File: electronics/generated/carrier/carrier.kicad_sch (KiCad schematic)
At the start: 11 parts, among them J1 EXTERNAL_3V3_CURRENT_LIMITED, J2 SPI_BANK_0, J3 SPI_BANK_1, J4 SPI_BANK_2, J5 SPI_BANK_3, J6 ADXL355_3V3_MODULE, J7 ODOMETER_3V3_ONLY, U1 Raspberry_Pi_Pico_USB_powered

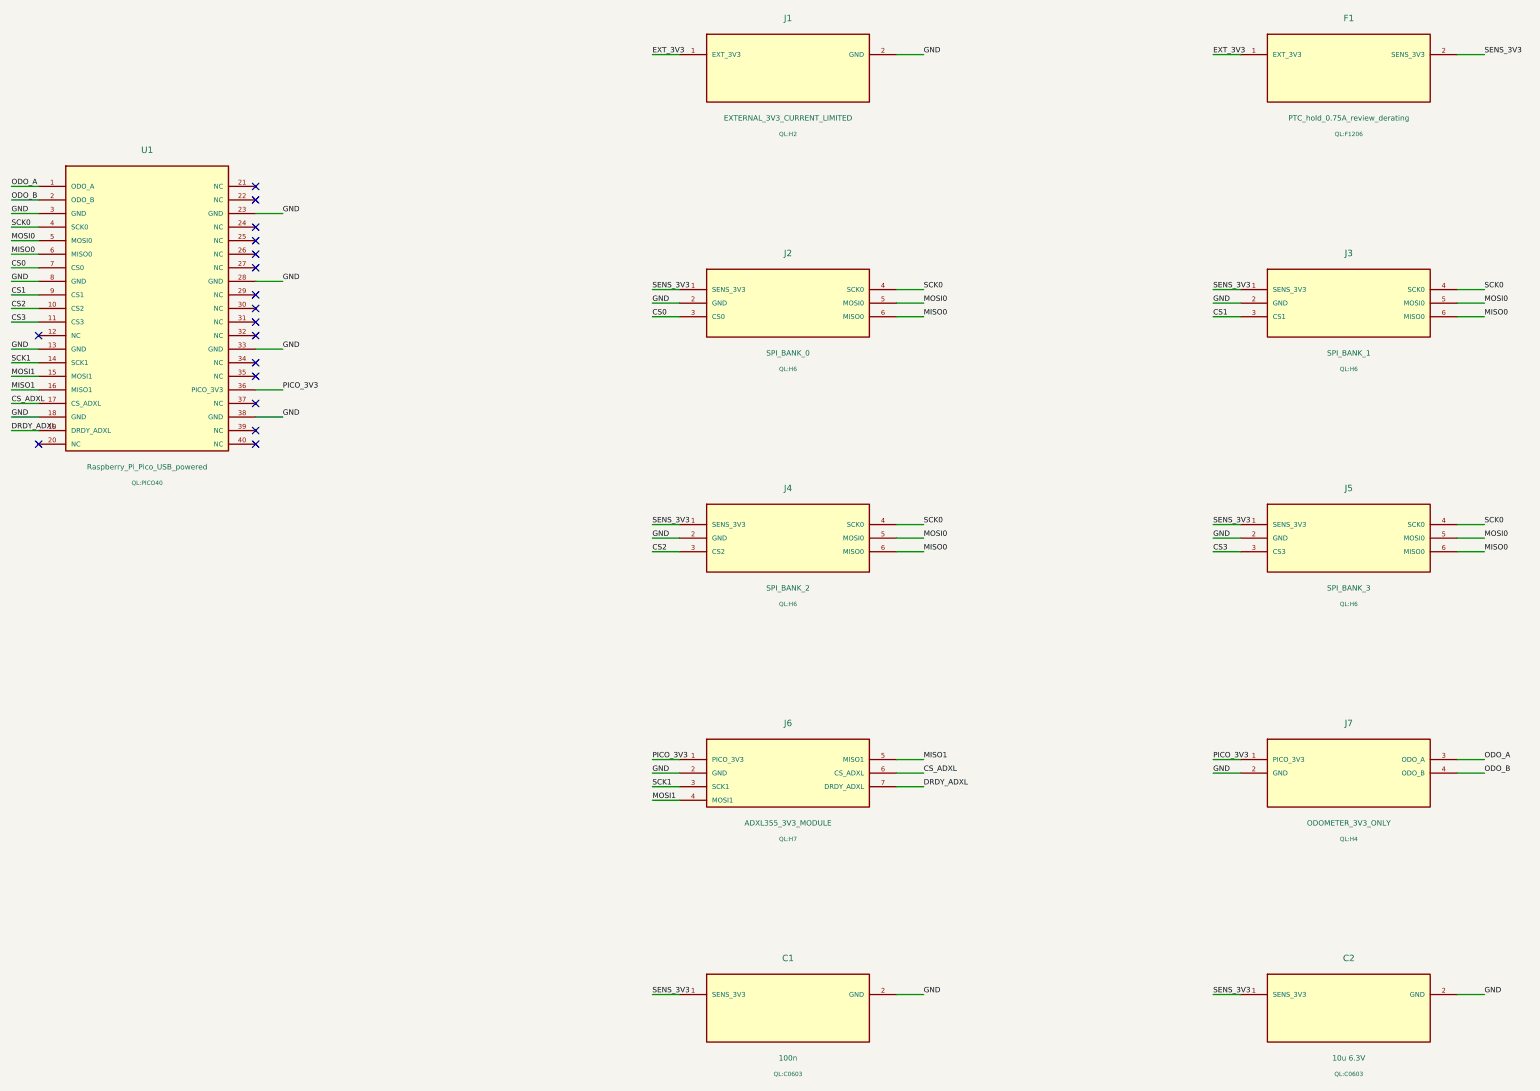
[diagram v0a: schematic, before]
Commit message: build: publish checked electronics/generated [skip ci]
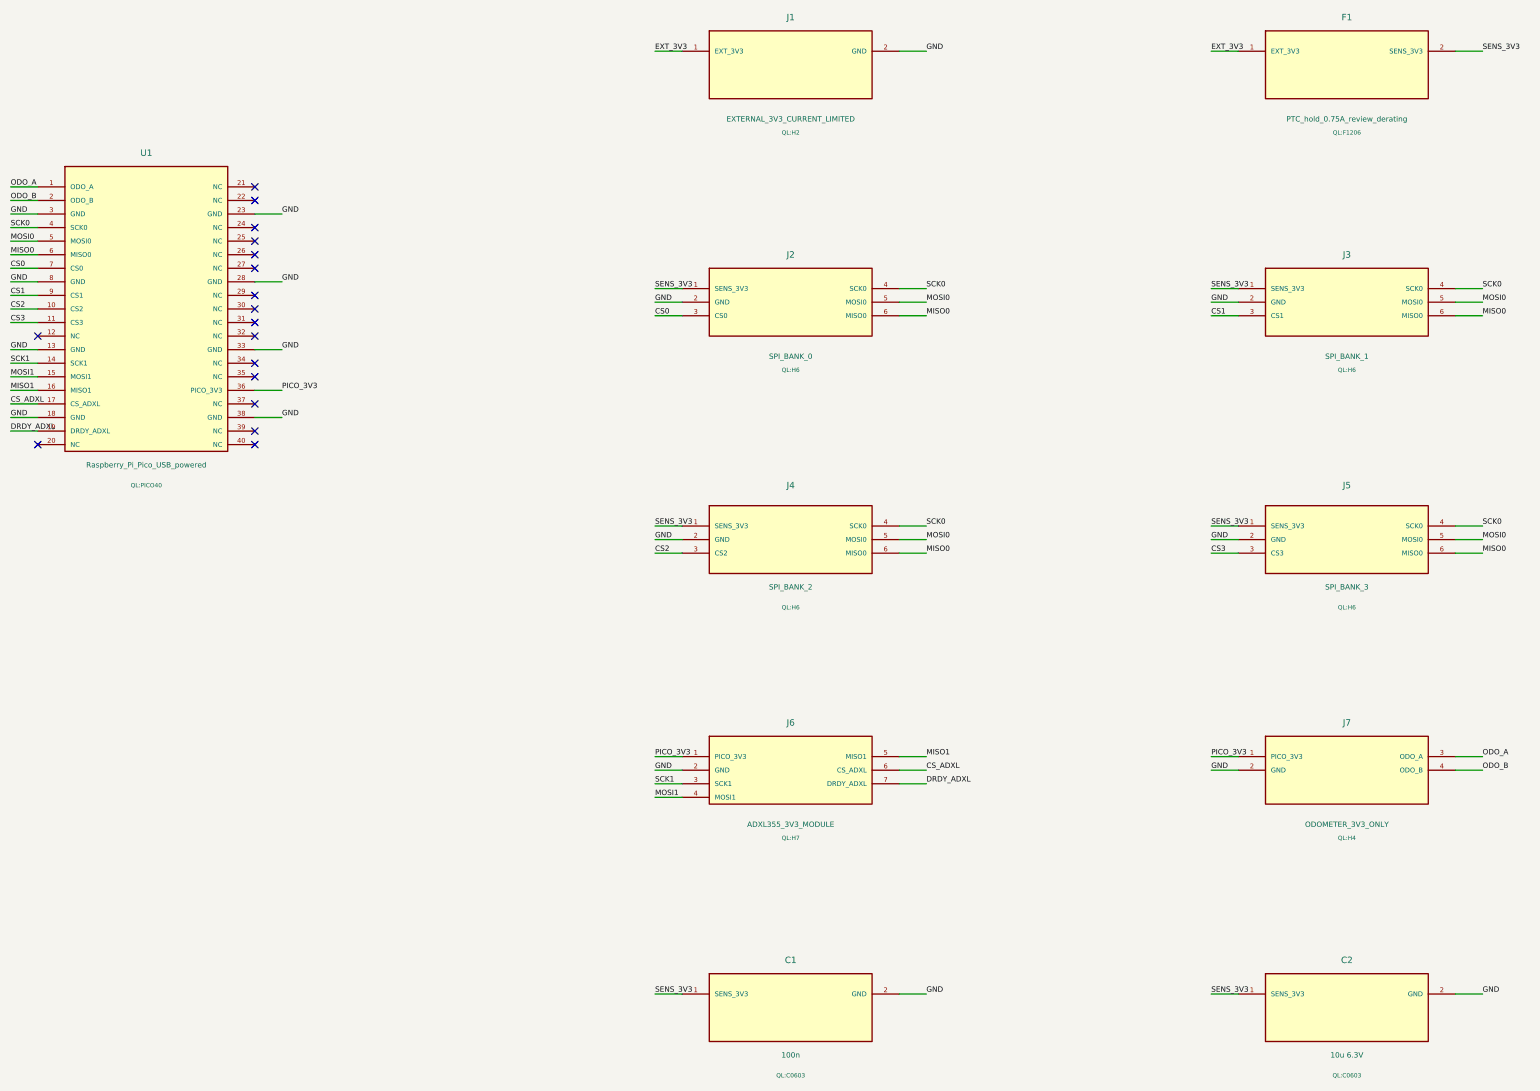
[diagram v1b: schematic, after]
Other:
- moved on the sheet: C1, F1, J1, J2, J4, J6, J7
